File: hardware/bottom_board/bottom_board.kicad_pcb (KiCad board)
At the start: 2 copper layers, 27.2 x 27.2 mm, 28 parts, among them IC1 74HC595, IC2 74HC595, J1 Conn_01x06_Socket, J2 Conn_01x06_Socket, Q1 Q_PNP_BCE, Q2 Q_PNP_BCE, Q3 Q_PNP_BCE, Q4 Q_PNP_BCE, Q5 Q_PNP_BCE, Q6 Q_PNP_BCE, SW1 SW_SPDT, U1 ATTINY1616-MNR, U2 LIS3DH

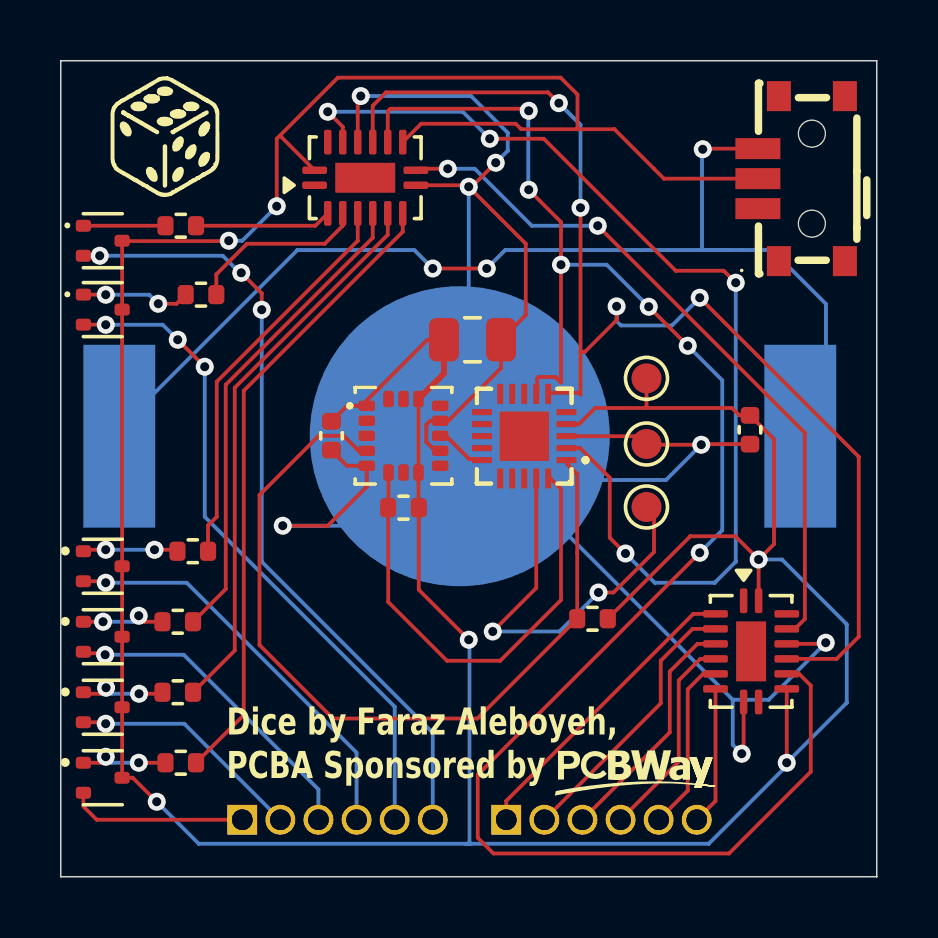
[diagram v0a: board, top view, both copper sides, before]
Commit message: Recent changes
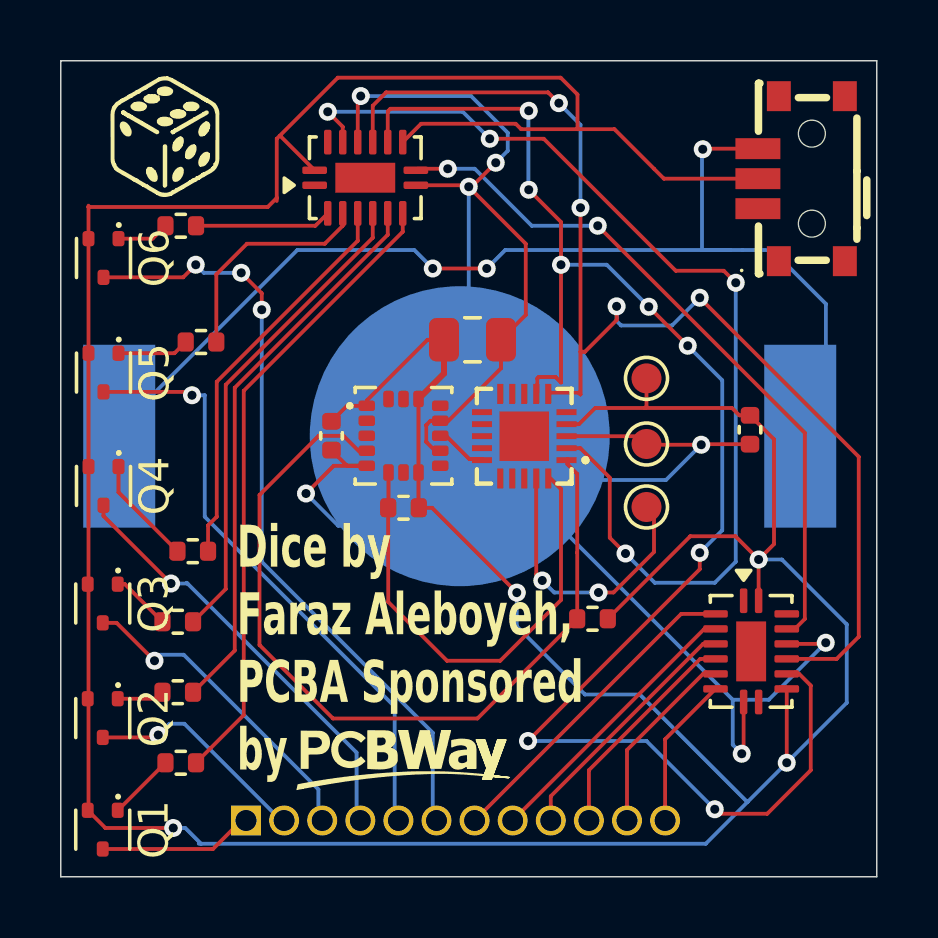
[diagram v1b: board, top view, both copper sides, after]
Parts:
- removed J2: Conn_01x06_Socket, Connector_PinSocket_1.27mm:PinSocket_1x06_P1.27mm_Vertical
- J1: value Conn_01x06_Socket -> Conn_01x12_Socket; footprint Connector_PinSocket_1.27mm:PinSocket_1x06_P1.27mm_Vertical -> Connector_PinSocket_1.27mm:PinSocket_1x12_P1.27mm_Vertical
- Q1, Q2, Q3, Q4, Q5, Q6: value Q_PNP_BCE -> Q_PNP_BEC
- R7, R8: value R -> 10k
- moved J1 8.68 mm to (95.2, 89.2)
- moved Q4 2.68 mm to (90.5, 78.0), turned to -90 degrees
- moved Q5 2.10 mm to (90.5, 74.3), turned to -90 degrees
- moved Q1 1.73 mm to (90.5, 89.5), turned to -90 degrees
- moved R5 1.58 mm to (93.8, 73.2)
- moved Q3 1.11 mm to (90.5, 82.0), turned to -90 degrees
- moved Q6 0.58 mm to (90.5, 70.5), turned to -90 degrees
- moved Q2 0.36 mm to (90.5, 85.8), turned to -90 degrees
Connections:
- J1 pad 1: /ROW1 -> /TO_Q1
- J1 pad 2: /ROW2 -> /TO_Q2
- J1 pad 3: /ROW3 -> /TO_Q3
- J1 pad 4: /ROW4 -> /TO_Q4
- J1 pad 5: /ROW5 -> /TO_Q5
- J1 pad 6: /ROW6 -> /TO_Q6
- Q1 pad 2: /TO_Q1 -> +3V0
- Q1 pad 3: +3V0 -> /TO_Q1
- Q2 pad 2: /TO_Q2 -> +3V0
- Q2 pad 3: +3V0 -> /TO_Q2
- Q3 pad 2: /TO_Q3 -> +3V0
- Q3 pad 3: +3V0 -> /TO_Q3
- Q4 pad 2: /TO_Q4 -> +3V0
- Q4 pad 3: +3V0 -> /TO_Q4
- Q5 pad 2: /TO_Q5 -> +3V0
- Q5 pad 3: +3V0 -> /TO_Q5
- Q6 pad 2: /TO_Q6 -> +3V0
- Q6 pad 3: +3V0 -> /TO_Q6
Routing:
- net +3V0: track 133.0 -> 140.2 mm, vias 6 -> 4
- net /SCLK: track 58.6 -> 53.3 mm, vias 6 -> 8
- net Net-(U1-PA0/~{RESET}/UPDI): track 13.8 -> 9.54 mm
- net /TO_Q5: track 22.3 -> 20.2 mm, vias 3 -> 1
- net GND: track 85.2 -> 83.3 mm
- net /COL5: track 5.97 -> 7.55 mm
- net Net-(Q5-B): track 3.66 -> 2.39 mm, vias 2 -> 0
- net Net-(Q2-B): track 2.80 -> 1.58 mm, vias 2 -> 0
- net Net-(Q6-B): track 2.73 -> 1.74 mm
- net /TO_Q1: track 5.93 -> 5.05 mm
- net Net-(Q3-B): track 2.80 -> 2.01 mm, vias 2 -> 0
- net /ROW1: track 10.2 -> 10.9 mm
- net /TO_Q4: track 13.7 -> 14.3 mm
- net Net-(Q4-B): track 3.35 -> 3.93 mm, vias 2 -> 0
- net /TO_Q6: track 26.6 -> 26.0 mm
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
